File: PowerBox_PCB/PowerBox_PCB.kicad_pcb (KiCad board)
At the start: 2 copper layers, 120 x 85 mm, 46 parts

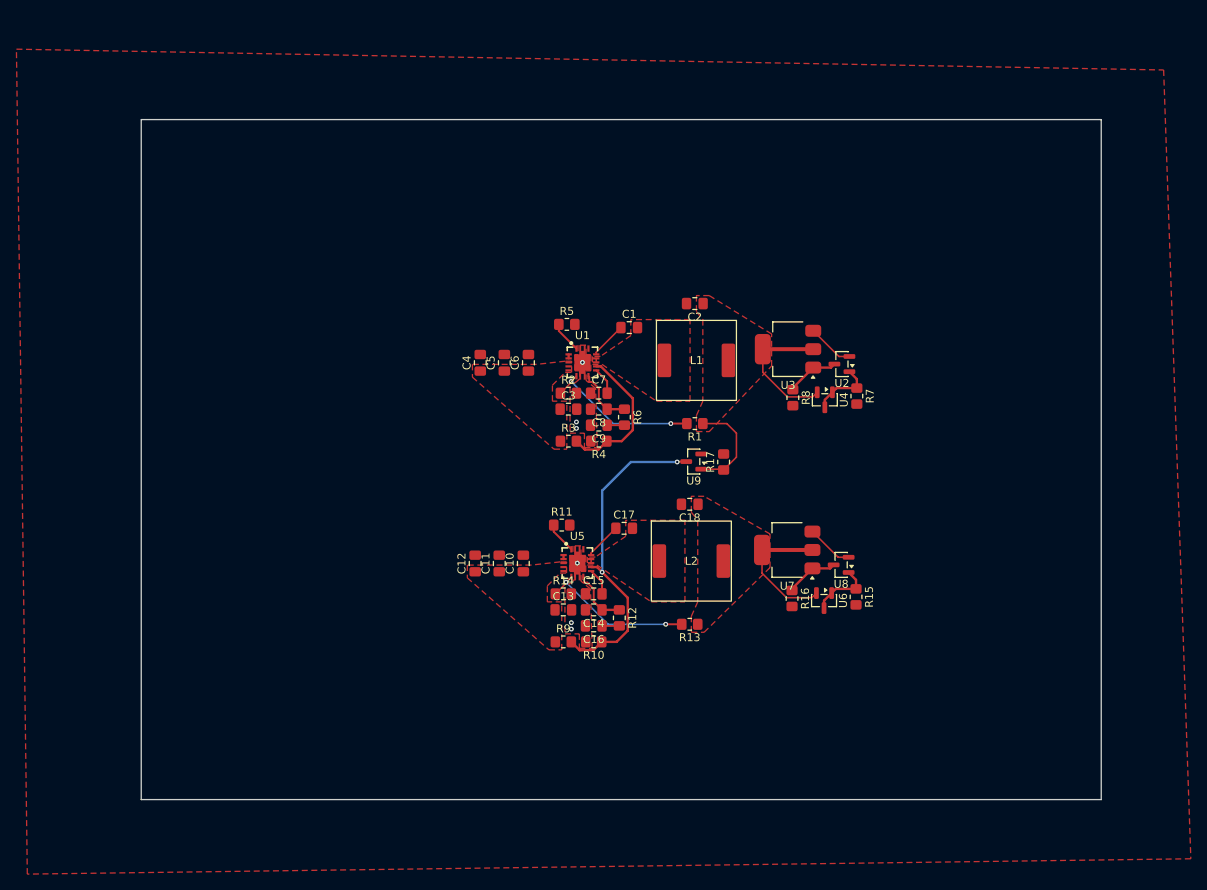
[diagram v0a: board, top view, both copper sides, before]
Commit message: Added USBPD & BMD & BATTCHARGER
Added USBPD & BMD & BATTCHARGER
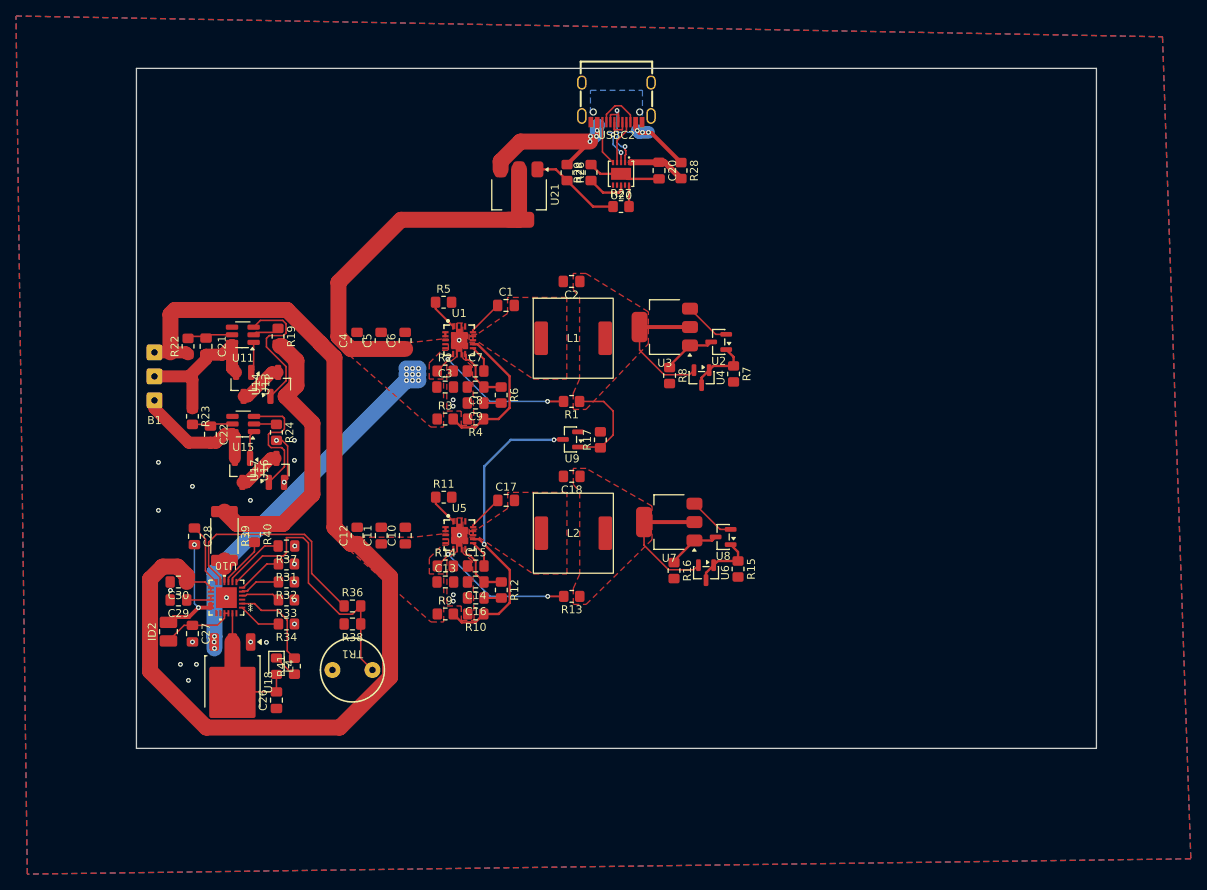
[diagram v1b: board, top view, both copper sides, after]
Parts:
- added B1: 2S Batt Pack, Custom_Footprints:2S Batt Pack, F.Cu at (52.2, 88.5)
- added C20: 1uF, Capacitor_SMD:C_0805_2012Metric_Pad1.18x1.45mm_HandSolder, F.Cu at (115.3, 62.8)
- added C21: 0.1uF, Capacitor_SMD:C_0805_2012Metric_Pad1.18x1.45mm_HandSolder, F.Cu at (58.7, 84.8)
- added C22: 0.1uF, Capacitor_SMD:C_0805_2012Metric_Pad1.18x1.45mm_HandSolder, F.Cu at (59.2, 95.8)
- added C26: 1uF, Capacitor_SMD:C_0805_2012Metric_Pad1.18x1.45mm_HandSolder, F.Cu at (67.5, 129.0)
- added C27: 10uf, Capacitor_SMD:C_0805_2012Metric_Pad1.18x1.45mm_HandSolder, F.Cu at (57.0, 120.7)
- added C28: 47nF, Capacitor_SMD:C_0805_2012Metric_Pad1.18x1.45mm_HandSolder, F.Cu at (57.2, 108.5)
- added C29: 44uF, Capacitor_SMD:C_0805_2012Metric_Pad1.18x1.45mm_HandSolder, F.Cu at (55.2, 116.5)
- added C30: 10uf, Capacitor_SMD:C_0805_2012Metric_Pad1.18x1.45mm_HandSolder, F.Cu at (55.2, 114.2)
- added ID2: 1uh, Inductor_SMD:L_1008_2520Metric_Pad1.43x2.20mm_HandSolder, F.Cu at (54.0, 120.4)
- added L4: LED, LED_SMD:LED_0805_2012Metric_Pad1.15x1.40mm_HandSolder, F.Cu at (67.5, 124.7)
- added R19: 1kΩ, Resistor_SMD:R_0805_2012Metric_Pad1.20x1.40mm_HandSolder, F.Cu at (67.7, 83.5)
- added R22: 100Ω, Resistor_SMD:R_0805_2012Metric_Pad1.20x1.40mm_HandSolder, F.Cu at (56.5, 84.8)
- added R23: 100Ω, Resistor_SMD:R_0805_2012Metric_Pad1.20x1.40mm_HandSolder, F.Cu at (57.0, 93.5)
- added R24: 1kΩ, Resistor_SMD:R_0805_2012Metric_Pad1.20x1.40mm_HandSolder, F.Cu at (67.5, 95.5)
- added R26: 49.9kΩ, Resistor_SMD:R_0805_2012Metric_Pad1.20x1.40mm_HandSolder, F.Cu at (103.8, 63.0)
- added R27: 5.1kΩ, Resistor_SMD:R_0805_2012Metric_Pad1.20x1.40mm_HandSolder, F.Cu at (110.6, 67.3)
- added R28: 10Ω, Resistor_SMD:R_0805_2012Metric_Pad1.20x1.40mm_HandSolder, F.Cu at (118.1, 62.8)
- added R29: 6.04Ω, Resistor_SMD:R_0805_2012Metric_Pad1.20x1.40mm_HandSolder, F.Cu at (106.8, 63.0)
- added R31: 10kΩ, Resistor_SMD:R_0805_2012Metric_Pad1.20x1.40mm_HandSolder, F.Cu at (68.8, 112.0)
- added R32: 10kΩ, Resistor_SMD:R_0805_2012Metric_Pad1.20x1.40mm_HandSolder, F.Cu at (68.8, 114.2)
- added R33: 10kΩ, Resistor_SMD:R_0805_2012Metric_Pad1.20x1.40mm_HandSolder, F.Cu at (68.8, 116.5)
- added R34: 10kΩ, Resistor_SMD:R_0805_2012Metric_Pad1.20x1.40mm_HandSolder, F.Cu at (68.8, 119.5)
- added R36: 5.23kΩ, Capacitor_SMD:C_0805_2012Metric_Pad1.18x1.45mm_HandSolder, F.Cu at (77.0, 117.2)
- added R37: 383Ω, Capacitor_SMD:C_0805_2012Metric_Pad1.18x1.45mm_HandSolder, F.Cu at (68.8, 109.7)
- added R38: 30.1kΩ, Capacitor_SMD:C_0805_2012Metric_Pad1.18x1.45mm_HandSolder, F.Cu at (77.0, 119.5)
- added R39: 10Ω_2W, Resistor_SMD:R_2512_6332Metric_Pad1.40x3.35mm_HandSolder, F.Cu at (61.0, 108.5)
- added R40: 300Ω, Resistor_SMD:R_0805_2012Metric_Pad1.20x1.40mm_HandSolder, F.Cu at (64.8, 108.2)
- added R41: 2.2kΩ, Resistor_SMD:R_0805_2012Metric_Pad1.20x1.40mm_HandSolder, F.Cu at (69.8, 124.7)
- added TR1: 10kΩ, Custom_Footprints:ThermistorPads, F.Cu at (77.0, 125.2)
- added U10: BQ25887RGER, BQ25887RGER:VQFN24_RGE_TEX, F.Cu at (61.2, 116.2)
- added U11: ~, Package_TO_SOT_SMD:SOT-23-6_Handsoldering, F.Cu at (63.3, 83.3)
- added U13: ~, Package_TO_SOT_SMD:SOT-23_Handsoldering, F.Cu at (63.4, 89.5)
- added U14: ~, Package_TO_SOT_SMD:SOT-23_Handsoldering, F.Cu at (67.7, 89.5)
- added U15: ~, Package_TO_SOT_SMD:SOT-23-6_Handsoldering, F.Cu at (63.4, 94.5)
- added U16: ~, Package_TO_SOT_SMD:SOT-23_Handsoldering, F.Cu at (63.2, 100.2)
- added U17: ~, Package_TO_SOT_SMD:SOT-23_Handsoldering, F.Cu at (67.5, 100.2)
- added U18: ~, Package_TO_SOT_SMD:TO-252-3_TabPin2, F.Cu at (62.0, 126.7)
- added U20: ~, Custom_Footprints:DFN-10_L3.0-W3.0-P0.50-BL-EP2.5, F.Cu at (110.6, 63.2)
- added U21: ~, Package_TO_SOT_SMD:SOT-223, F.Cu at (97.8, 65.8)
- added USBC2: ~, Custom_Footprints:USB-C_SMD-TYPE-C-31-M-12_1, F.Cu at (110.0, 54.2)
- moved R7 15.7 mm to (124.6, 88.2)
- moved R8 15.7 mm to (116.6, 88.4)
- moved U4 15.7 mm to (120.6, 88.7)
- moved C1 15.7 mm to (96.2, 79.6)
- moved C2 15.7 mm to (104.4, 76.6)
- moved C3 15.7 mm to (88.6, 89.8)
- moved C4 15.7 mm to (77.6, 84.0)
- moved C5 15.7 mm to (80.6, 84.0)
- moved C6 15.7 mm to (83.6, 84.0)
- moved C7 15.7 mm to (92.4, 87.8)
- moved C8 15.7 mm to (92.4, 89.8)
- moved C9 15.7 mm to (92.4, 91.8)
- moved L1 15.7 mm to (104.6, 83.7)
- moved R1 15.7 mm to (104.4, 91.6)
- moved R17 15.7 mm to (108.0, 96.4)
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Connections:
- net /TPS54620_Buck/VIN_BUCK renamed VUSBPD
- net /TPS54620_Buck1/VIN_BUCK renamed P+
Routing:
- net P+: track 0.00 -> 133.2 mm
- net VUSBPD: track 0.00 -> 95.8 mm, vias 0 -> 12
- net /Batt Charger/TS: track 0.00 -> 34.9 mm
- net PM: track 0.00 -> 34.6 mm
- net /USBPD/VBUS: track 0.00 -> 33.8 mm, vias 0 -> 7
- net Net-(U10-REGN): track 0.00 -> 29.0 mm
- net /BMS/BM: track 0.00 -> 19.7 mm
- net /Batt Charger/VOUT: track 0.00 -> 17.6 mm
- net Net-(U11-OC): track 0.00 -> 17.5 mm
- net /BMS/B-: track 0.00 -> 16.5 mm
- net Net-(U15-OC): track 0.00 -> 15.9 mm
- net GND: track 1.00 -> 16.7 mm, vias 6 -> 27
- net /Batt Charger/SW: track 0.00 -> 14.9 mm, vias 0 -> 2
- net /USBPD/D+: track 0.00 -> 11.7 mm, vias 0 -> 2
- net Net-(U10-STAT): track 0.00 -> 11.6 mm
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- added copper zone on B.Cu, net /USBPD/VBUS
- added copper zone on B.Cu, net GND
